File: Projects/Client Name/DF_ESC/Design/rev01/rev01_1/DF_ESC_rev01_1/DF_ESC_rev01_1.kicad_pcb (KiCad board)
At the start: 4 copper layers, 100 x 75 mm, 187 parts, among them J1 XT60PW-M, J2 HX25003-8AWB, J3 S6B-XH-SM4-TB(LF)(SN), J4 XH-3AWB, J5 7461084, J6 7461084, J7 7461084, J8 USB_C_Receptacle_USB2.0, Q1 HSBA15810C, Q2 HSBA15810C, Q3 HSBA15810C, Q4 HSBA15810C, Q5 HSBA15810C, Q6 HSBA15810C, SW1 SW_DIP_x01, U1 XH-2PWBPZ, U10 PUSB3AB6Z, U2 AMS1117-3.3, U3 STM32F405RGTx, U4 DRV8302DCAR, U5 S4B-XH-SM4-TB-(LF)(SN), U6 ESDCAN24-2BLY, U7 744227S, U8 SN65HVD230, U9 S6B-XH-SM4-TB(LF)(SN), Y1 Crystal_Small

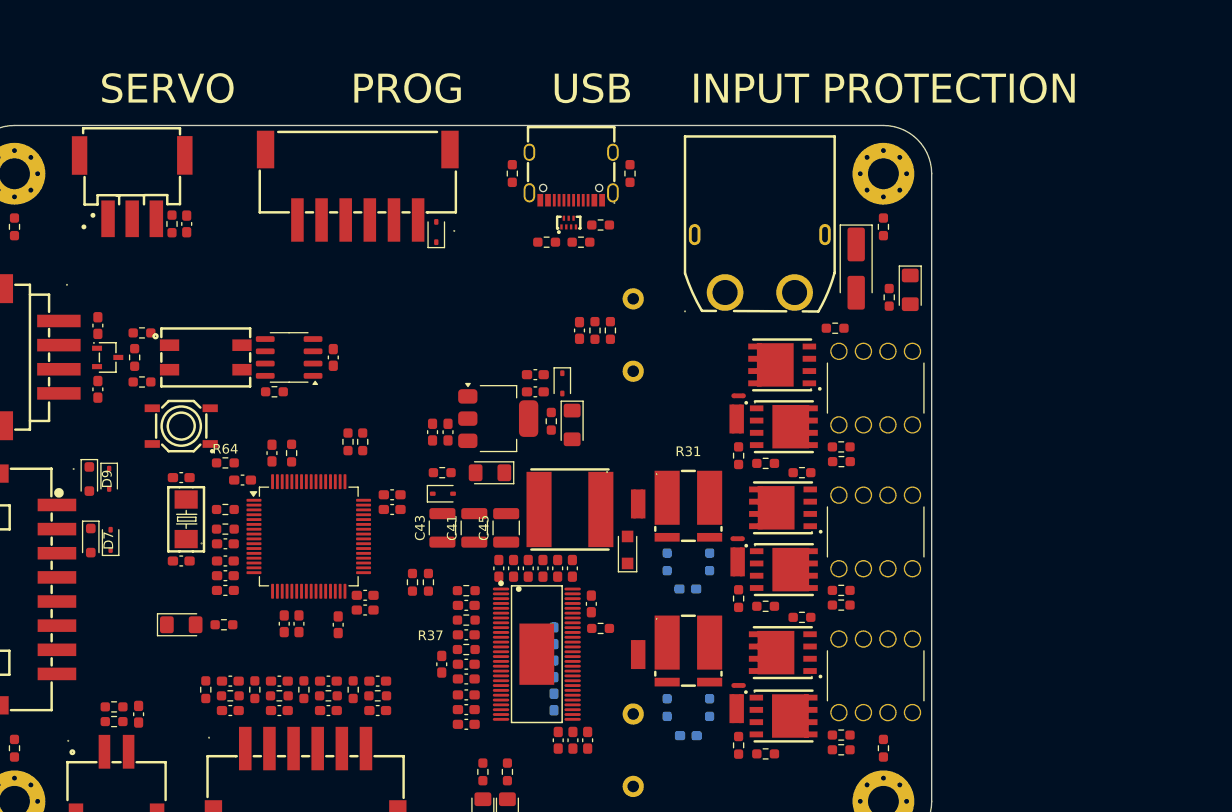
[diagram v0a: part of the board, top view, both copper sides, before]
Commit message: update 2024-04-18
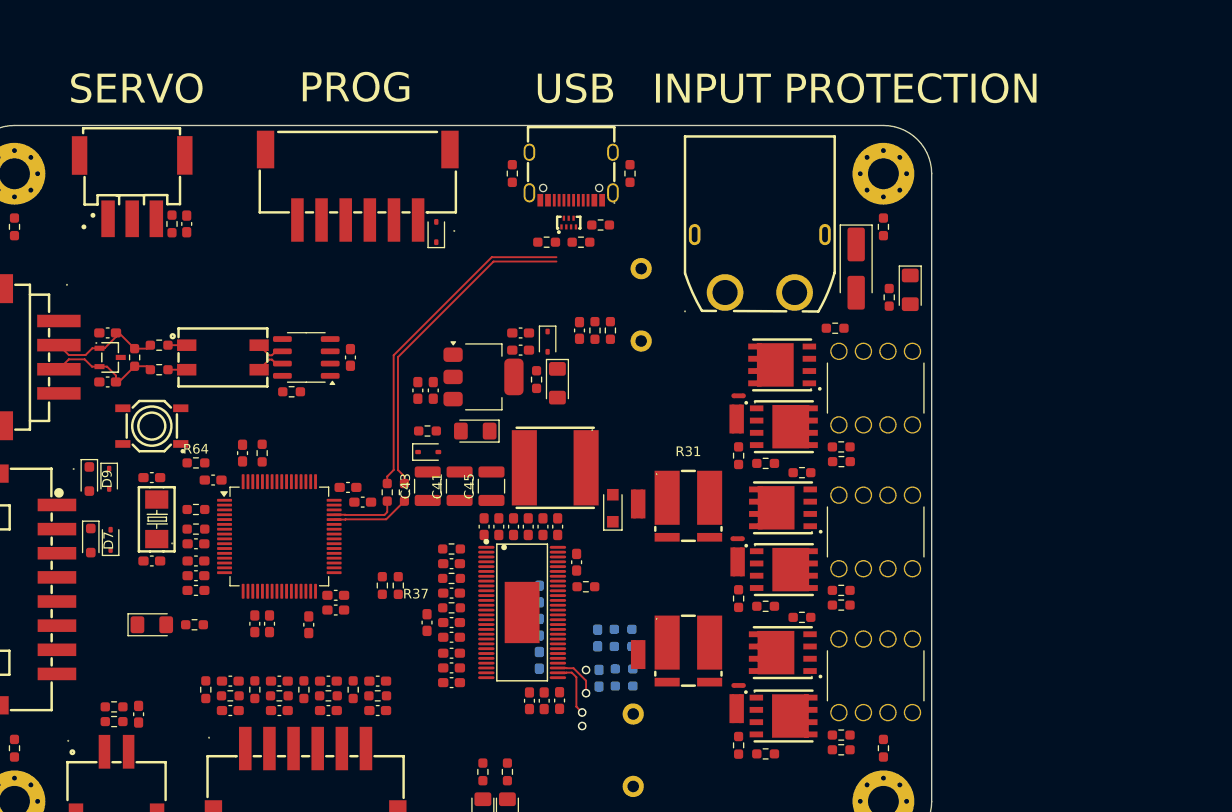
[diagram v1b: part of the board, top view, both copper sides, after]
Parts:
- moved R28 12.5 mm to (251.9, 150.1), turned to 0 degrees
- moved C49 11.0 mm to (249.4, 153.4), turned to 90 degrees
- moved C48 10.6 mm to (249.2, 149.2), turned to 90 degrees
- moved R34 9.13 mm to (252.0, 154.2), turned to 0 degrees
- moved R29 8.34 mm to (251.9, 148.3), turned to 0 degrees
- moved R58 7.84 mm to (229.2, 134.1)
- moved R35 5.99 mm to (252.0, 152.4), turned to 0 degrees
- moved R59 5.81 mm to (227.4, 134.1)
- moved C33 5.06 mm to (242.2, 155.7)
- moved C35 5.06 mm to (243.7, 155.7)
- moved C32 5.04 mm to (245.3, 155.7)
- moved C11 4.64 mm to (223.4, 133.6)
- moved C24 4.58 mm to (234.1, 150.8)
- moved C27 4.58 mm to (234.1, 152.3)
- moved C31 4.58 mm to (234.1, 153.8)
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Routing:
- net /[9] - USB/USB-C_P: track 0.00 -> 34.6 mm
- net /[9] - USB/USB-C_N: track 0.00 -> 33.9 mm
- net /[7] - CAN/C_CAN_P: track 0.00 -> 12.1 mm
- net /[7] - CAN/C_CAN_N: track 0.00 -> 11.9 mm
- net USB_N: track 0.00 -> 8.07 mm
- net USB_P: track 0.00 -> 6.77 mm
- net S2_P: track 0.00 -> 6.03 mm, vias 0 -> 1
- net S2_N: track 0.00 -> 4.82 mm, vias 0 -> 1
- net /[7] - CAN/CAN_P: track 0.00 -> 3.01 mm
- net /[7] - CAN/CAN_N: track 0.00 -> 3.01 mm
- net /[7] - CAN/R_CAN_P: track 0.00 -> 1.94 mm
- net /[7] - CAN/R_CAN_N: track 0.00 -> 1.94 mm
- net GND: vias 0 -> 2

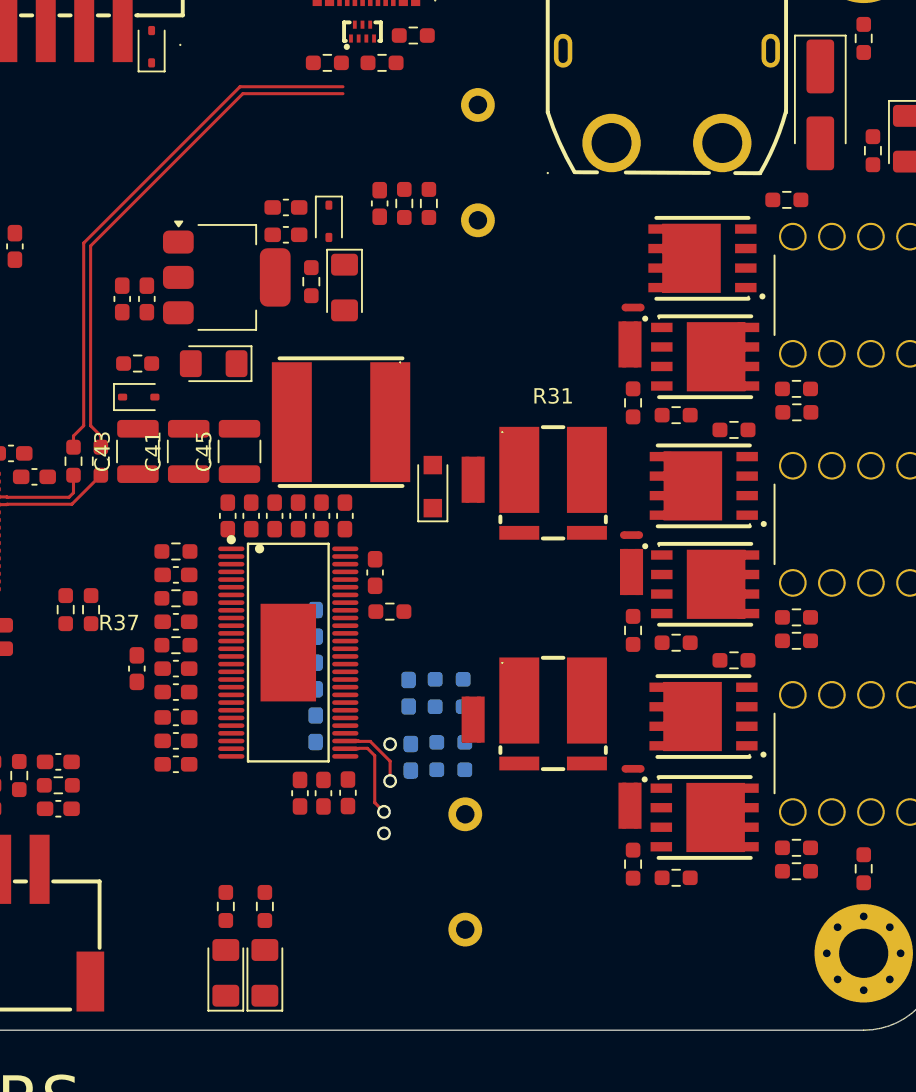
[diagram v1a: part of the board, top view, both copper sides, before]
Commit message: update 20240419
preliminari Routing
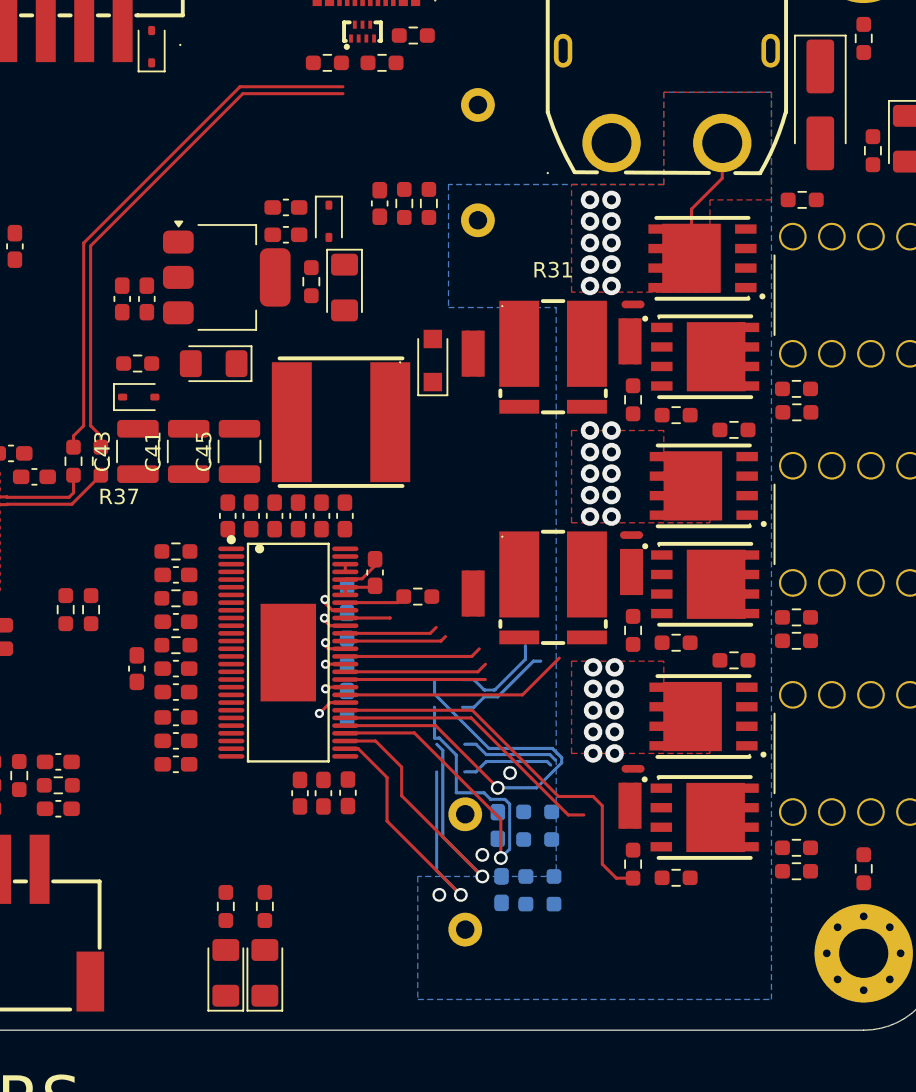
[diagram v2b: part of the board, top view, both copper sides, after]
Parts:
- moved R35 12.0 mm to (257.8, 162.9)
- moved R29 11.9 mm to (257.6, 158.7)
- moved C49 10.4 mm to (255.3, 162.0), turned to -90 degrees
- moved C48 10.4 mm to (255.0, 157.8), turned to -90 degrees
- moved R34 9.04 mm to (257.8, 161.1)
- moved R28 8.94 mm to (257.6, 156.9)
- moved R31 8.20 mm to (258.6, 127.3)
- moved R37 8.20 mm to (258.6, 142.3)
- moved D14 8.20 mm to (250.8, 127.6)
- moved NT5 8.20 mm to (253.4, 142.7)
- moved NT8 8.20 mm to (253.4, 127.1)
- moved C46 2.59 mm to (245.2, 149.9)
- moved C42 2.57 mm to (245.2, 146.5)
- moved C39 2.56 mm to (245.2, 143.1)
- moved R17 2.06 mm to (249.8, 142.9)
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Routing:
- net S1_P: track 0.00 -> 28.8 mm, vias 0 -> 1
- net S1_N: track 0.00 -> 27.7 mm, vias 0 -> 1
- net M_L3: track 0.00 -> 25.5 mm
- net S2_N: track 4.82 -> 23.5 mm
- net H3_LOW: track 0.00 -> 18.1 mm
- net S2_P: track 6.03 -> 21.8 mm
- net M_H3: track 0.00 -> 14.9 mm
- net M_L2: track 0.00 -> 9.32 mm
- net H2_LOW: track 0.00 -> 9.11 mm
- net M_H2: track 0.00 -> 8.92 mm
- net +VDC: track 0.00 -> 8.83 mm, vias 0 -> 30
- net H1_LOW: track 0.00 -> 6.64 mm
- net /[6] - MOSFETs/SH2_N: track 0.00 -> 6.34 mm
- net /[6] - MOSFETs/SH1_P: track 0.00 -> 6.33 mm
- net M_L1: track 0.00 -> 6.08 mm
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- added copper zone on B.Cu, net +VDC
- added copper zone on F.Cu, net +VDC
